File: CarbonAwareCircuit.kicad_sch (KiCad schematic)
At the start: 11 parts, among them J1 USB_C_Receptacle_USB2.0_14P, SW1 SW_Push_Dual_x2, SW2 SW_Push_Dual_x2, U1 LD1117V33, U2 ESP32-C3-WROOM-02

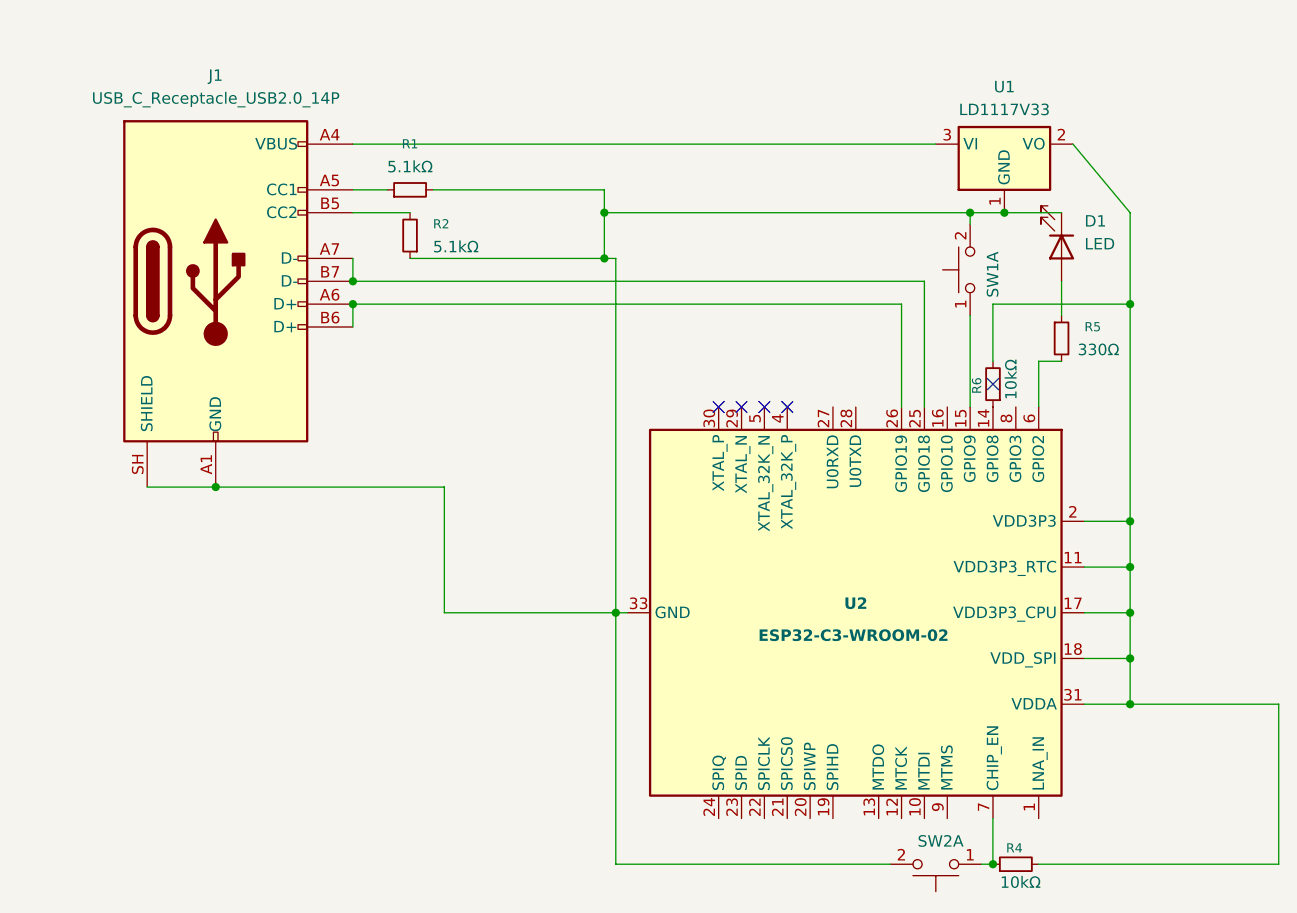
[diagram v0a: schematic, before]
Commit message: decided to restart :(
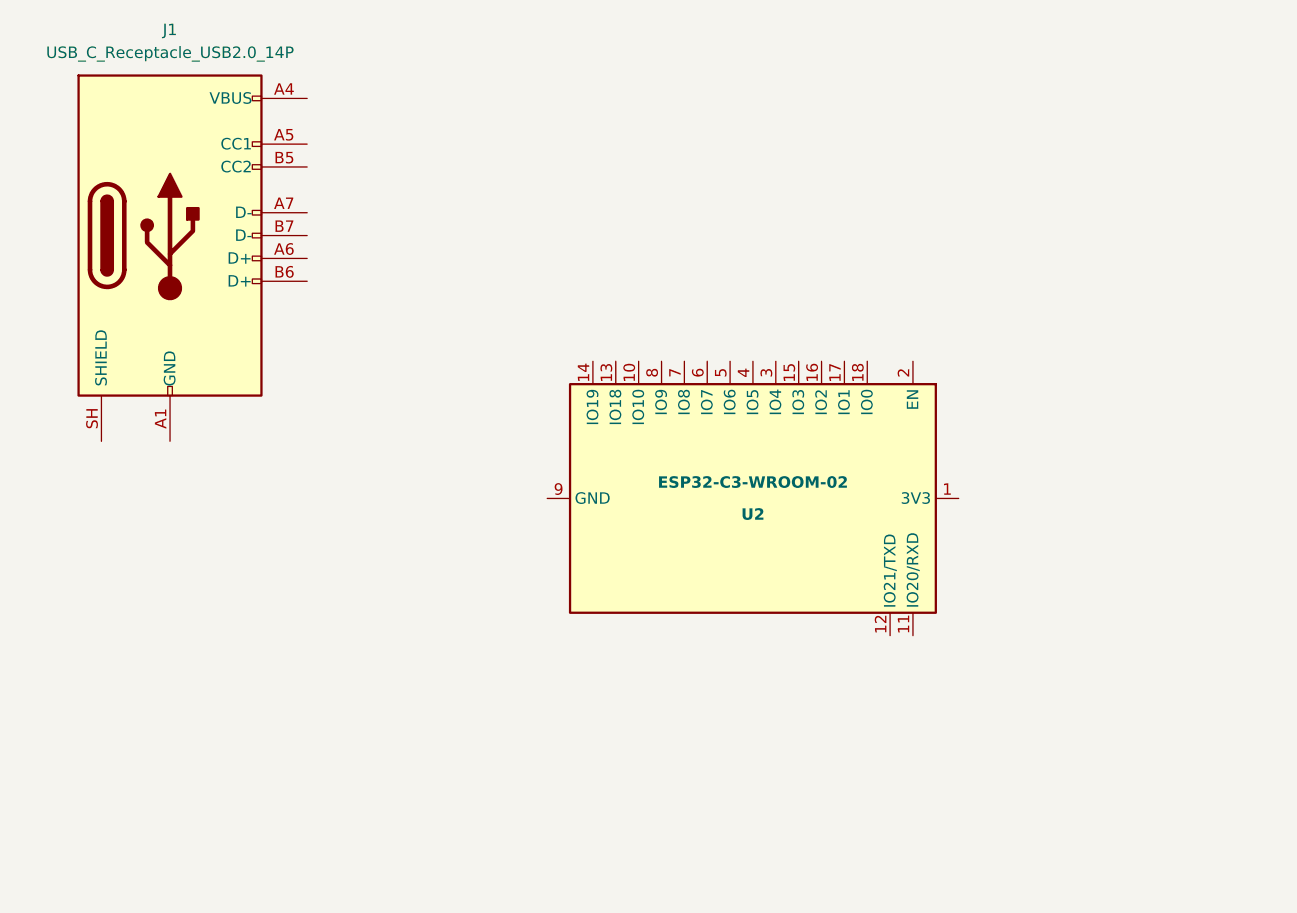
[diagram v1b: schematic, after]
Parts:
- removed D1: LED, LED_THT:LED_D2.0mm_W4.8mm_H2.5mm_FlatTop, symbol Device:LED
- removed R1: 5.1kΩ, Resistor_THT:R_Axial_DIN0309_L9.0mm_D3.2mm_P25.40mm_Horizontal, symbol Device:R_Small
- removed R2: 5.1kΩ, Resistor_THT:R_Axial_DIN0411_L9.9mm_D3.6mm_P5.08mm_Vertical, symbol Device:R_Small
- removed R4, R6: 10kΩ, Resistor_THT:R_Axial_DIN0411_L9.9mm_D3.6mm_P5.08mm_Vertical, symbol Device:R_Small
- removed R5: 330Ω, Resistor_THT:R_Axial_DIN0411_L9.9mm_D3.6mm_P5.08mm_Vertical, symbol Device:R_Small
- removed SW1: SW_Push_Dual_x2, Button_Switch_THT:SW_DIP_SPSTx05_Piano_CTS_Series194-5MSTN_W7.62mm_P2.54mm, symbol Switch:SW_Push_Dual_x2
- removed SW2: SW_Push_Dual_x2, Button_Switch_THT:SW_DIP_SPSTx03_Piano_10.8x9.18mm_W7.62mm_P2.54mm, symbol Switch:SW_Push_Dual_x2
- removed U1: LD1117V33, Package_TO_SOT_THT:TO-220-3_Vertical, symbol Regulator_Linear:LD1117V33
- removed U2: ESP32-C3-WROOM-02, Package_DFN_QFN:QFN-32-1EP_5x5mm_P0.5mm_EP3.7x3.7mm, symbol MCU_Espressif:ESP32-C3
- added U2: ESP32-C3-WROOM-02, RF_Module:ESP32-C3-WROOM-02, symbol RF_Module:ESP32-C3-WROOM-02
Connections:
- net at J1.A1 (GND), J1.A12 (GND), J1.B1 (GND)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: no longer J1.SH (SHIELD)
- net at J1.A6 (D+): no longer J1.B6 (D+)
- net at J1.A7 (D-): no longer J1.B7 (D-)
- new net: U2.19 (GND), U2.9 (GND)
- no-connect marks 5 -> 0
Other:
- moved on the sheet: J1
